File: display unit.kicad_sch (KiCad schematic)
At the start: 1 part

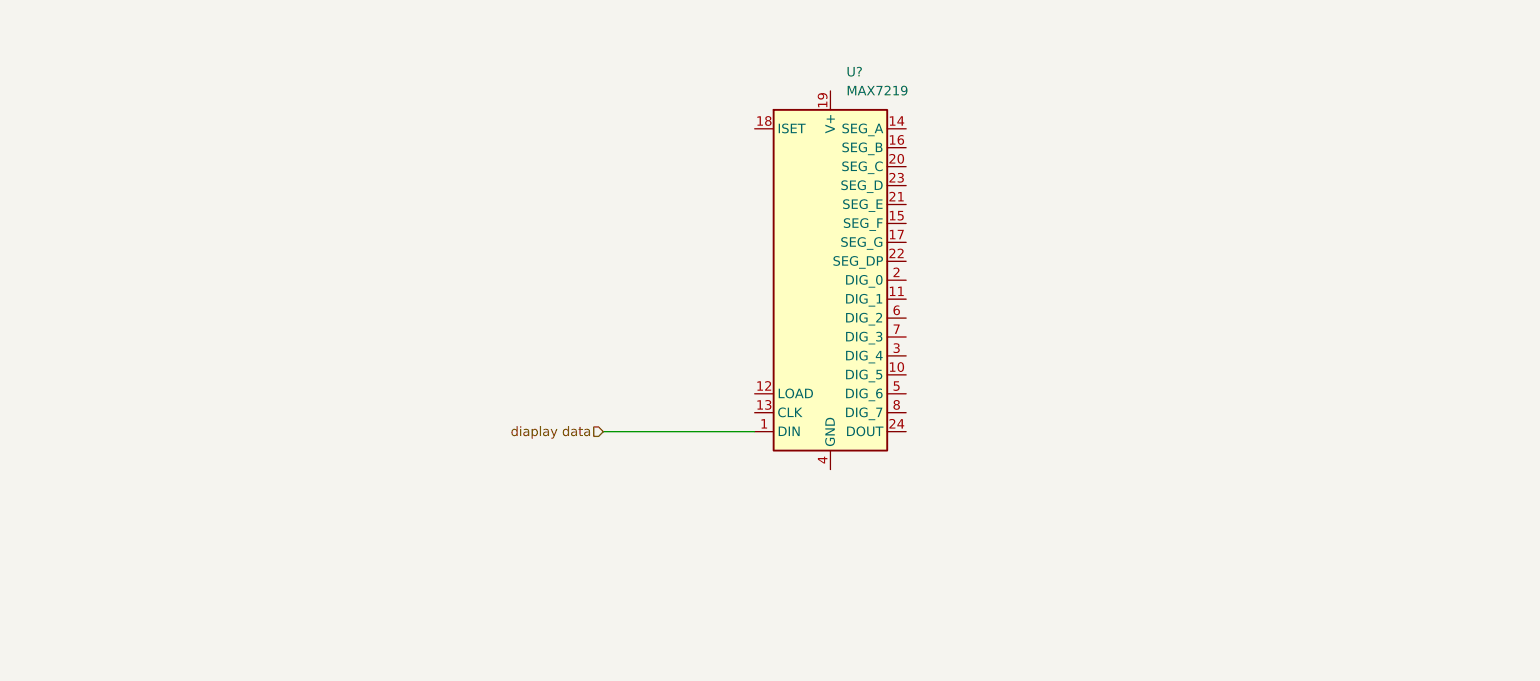
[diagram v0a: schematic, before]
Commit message: disp changes
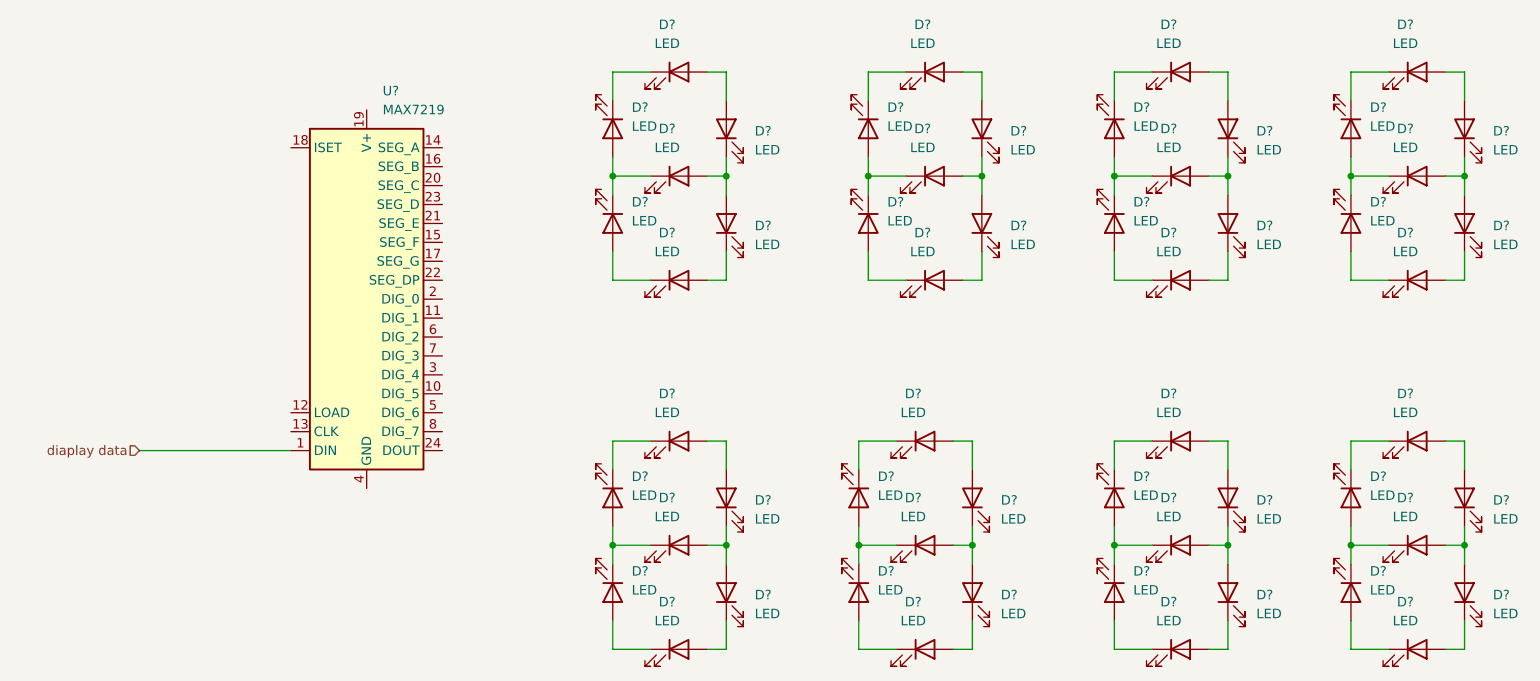
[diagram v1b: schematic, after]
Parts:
- added D? (x56): LED, symbol Device:LED
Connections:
- new net: D?.1 (K), D?.2 (A) (x16)
- new net: D?.1 (K), D?.2 (A), D?.2 (A) (x8)
- new net: D?.1 (K), D?.1 (K) (x8)
- new net: D?.2 (A), D?.2 (A) (x8)
- new net: D?.1 (K), D?.1 (K), D?.2 (A) (x8)
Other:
- moved on the sheet: U?
